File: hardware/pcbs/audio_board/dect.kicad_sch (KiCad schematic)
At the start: 1 part, among them J9 DECT

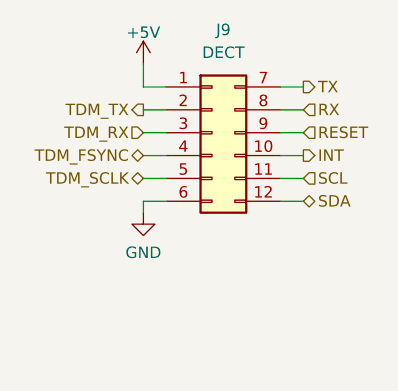
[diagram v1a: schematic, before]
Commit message: routing almost complete
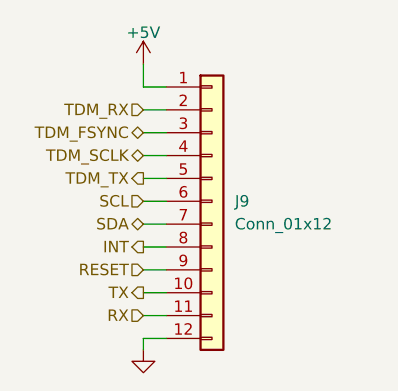
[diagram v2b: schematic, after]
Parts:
- removed J9: DECT, extra:DectModule, symbol Connector_Generic:Conn_02x06_Top_Bottom
- added J9: Conn_01x12, Connector_PinHeader_2.54mm:PinHeader_1x12_P2.54mm_Vertical, symbol Connector_Generic:Conn_01x12
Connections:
- net +5V: now also J9.1 (Pin_1)
- net GND: now also J9.12 (Pin_12)
- net INT: now also J9.8 (Pin_8)
- net RESET: now also J9.9 (Pin_9)
- net RX: now also J9.11 (Pin_11)
- net SCL: now also J9.6 (Pin_6)
- net SDA: now also J9.7 (Pin_7)
- net TDM_FSYNC: now also J9.3 (Pin_3)
- net TDM_RX: now also J9.2 (Pin_2)
- net TDM_SCLK: now also J9.4 (Pin_4)
- net TDM_TX: now also J9.5 (Pin_5)
- net TX: now also J9.10 (Pin_10)
